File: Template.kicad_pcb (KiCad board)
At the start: 2 copper layers, 62 x 62 mm, 154 parts, among them J10 TAG, J20 TAG, J50 Goldpin, J60 RS232_Power, J61 RS232_Data, J70 USB, J84 Key, J86 Key, J87 Key, J90 12VIN, K85 CONFIG, T80 BC847, T81 BC847, T82 BC847, T83 BC847, T84 BC847, T90 BC847, U10 ATmega4809-MFR, U20 ATSAMW25-MR210PB, U30 ATECC608A-SSHDA, U31 ATECC608A-MAHDA, U40 GD25Q64C, U60 MAX3232, U70 FT230XQ, U90 AP3211, U91 1117-3.3, X10 32768Hz

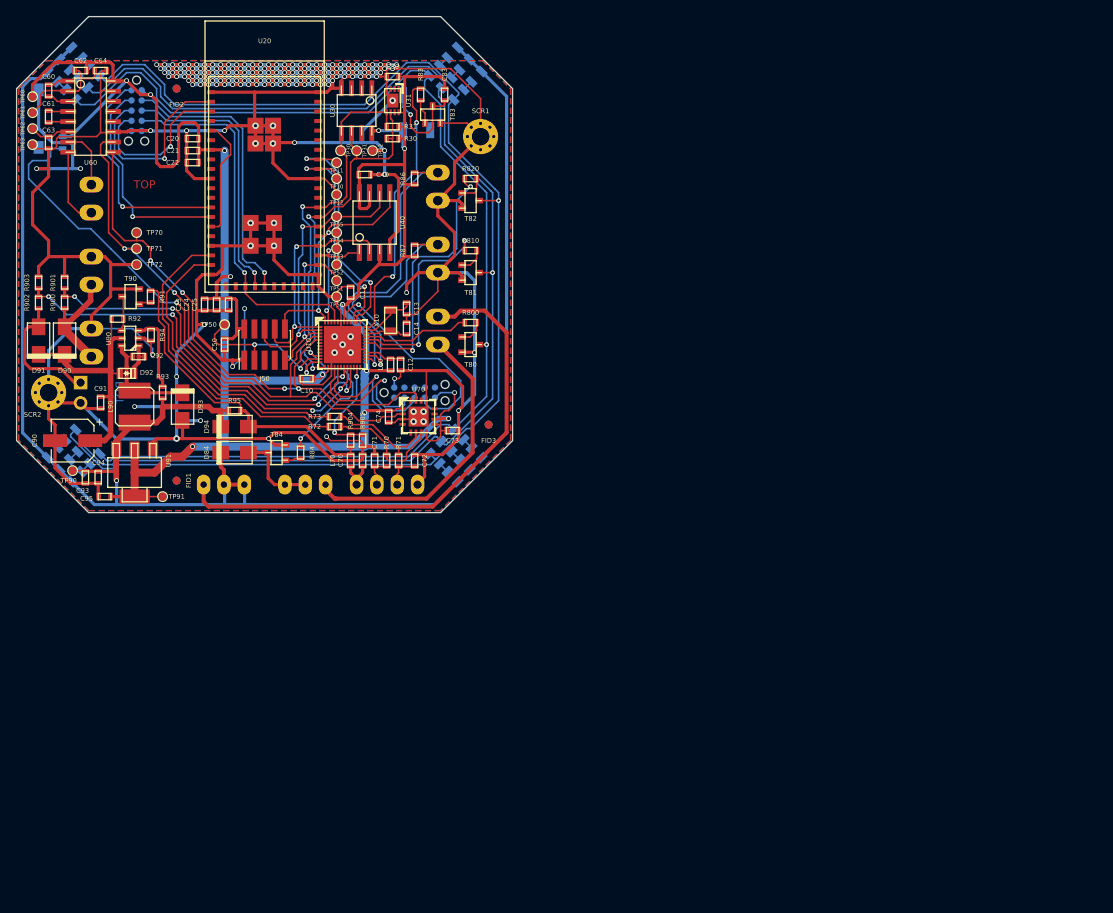
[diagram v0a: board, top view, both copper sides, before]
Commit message: Testowa modyfikacja
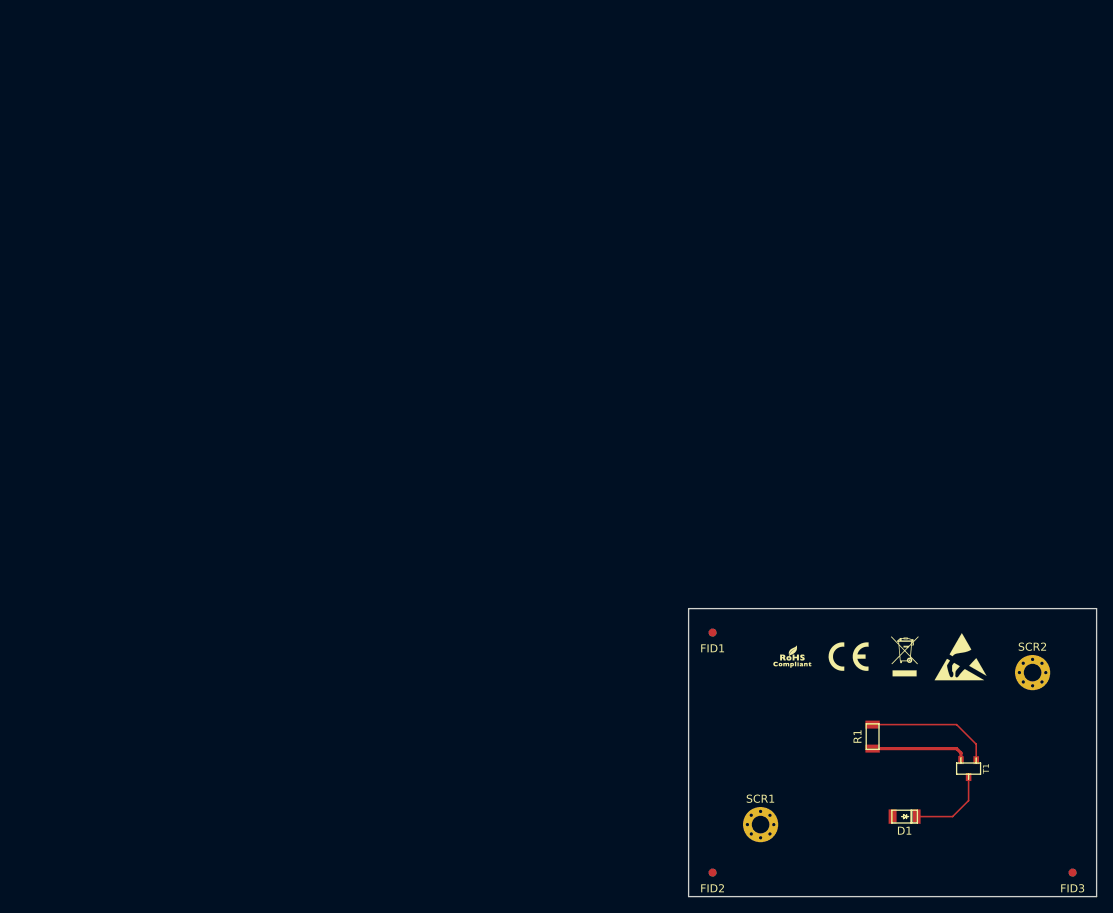
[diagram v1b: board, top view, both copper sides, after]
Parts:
- removed BT90: BATTERY, Pin_Headers:Pin_Header_Straight_1x02_Pitch2.54mm
- removed C10, C11, C12, C20, C23, C30, C50, C60, C61, C62, C63, C64, C70, C73, C74, C83, C94: 100n, _obudowy:C_0603
- removed C13, C14, C40: 15p, _obudowy:C_0603
- removed C21, C24: 1u, _obudowy:C_0603
- removed C22, C25, C93, C95: 10u, _obudowy:C_0603
- removed C71, C72: 22p, _obudowy:C_0603
- removed C90: 10u/50V, Capacitors_SMD:CP_Elec_5x5.8
- removed C91: 100n/50V, _obudowy:C_0603
- removed C92: 10n, _obudowy:C_0603
- removed D801, D802, D803, D804: Red, _obudowy:LED_0805
- removed D811, D812, D813, D814: Green, _obudowy:LED_0805
- removed D821, D822, D823, D824: Blue, _obudowy:LED_0805
- removed D84, D90, D91, D93, D94: SS14, _obudowy:D_SMA_DO214AC
- removed D92: 1N4148, _obudowy:D_0805
- removed G***: LOGO, _obudowy:SafliLogo
- removed J10, J20: TAG, _obudowy:TAG-TC2050
- removed J50: Goldpin, Pin_Headers:Pin_Header_Straight_2x05_Pitch1.27mm_SMD
- removed J60: RS232_Power, _obudowy:ADAM_TECH_EB59A-1-02-A-R
- removed J61: RS232_Data, _obudowy:ADAM_TECH_EB59A-1-02-A-R
- removed J70: USB, Pin_Headers:Pin_Header_Straight_1x04_Pitch2.54mm
- removed J84, J86, J87: Key, _obudowy:ADAM_TECH_EB59A-1-02-A-R
- removed J90: 12VIN, _obudowy:ADAM_TECH_EB59A-1-02-A-R
- removed K85: CONFIG, _obudowy:TACT_6x3.5_SMD
- removed L10, L70: BLM18PG471SN1, _obudowy:L_0603
- removed L90: 4.7uH, _obudowy:DJNR4018-5020
- removed R30, R31, R85, R86, R87, R901, R903, R904, R905, R91: 10k, _obudowy:R_0603
- removed R70, R71: 22R, _obudowy:R_0603
- removed R72, R73, R95: 0R, _obudowy:R_0603
- removed R800, R810, R820, R83, R84: 1k, _obudowy:R_0603
- removed R801, R802, R803, R804, R811, R812, R813, R814, R821, R822, R823, R824: 220R, _obudowy:R_0805
- removed R900, R902: 100k, _obudowy:R_0603
- removed R92: 1M, _obudowy:R_0603
- removed R93: 27k, _obudowy:R_0603
- removed R94: 5k1, _obudowy:R_0603
- removed RY80: RayexR1, _obudowy:Relay-Rayex1357
- removed S83: LD-BZEL-T54-0505, _obudowy:Loudity-SMT54
- removed T80, T81, T82, T83, T84, T90: BC847, _obudowy:SOT23
- removed TP10: LinkRx, _obudowy:Testpoint_1.00mm
- removed TP11: LinkTx, _obudowy:Testpoint_1.00mm
- removed TP12, TP32, TP56, TP63, TP72: GND, _obudowy:Testpoint_1.00mm
- removed TP30: SDA, _obudowy:Testpoint_1.00mm
- removed TP31: SCL, _obudowy:Testpoint_1.00mm
- removed TP50: Reset-RFID, _obudowy:Testpoint_1.00mm
- removed TP51: CS-RFID, _obudowy:Testpoint_1.00mm
- removed TP52: CS-Flash, _obudowy:Testpoint_1.00mm
- removed TP53: MISO, _obudowy:Testpoint_1.00mm
- removed TP54: MOSI, _obudowy:Testpoint_1.00mm
- removed TP55: SCK, _obudowy:Testpoint_1.00mm
- removed TP60: Vcc, _obudowy:Testpoint_1.00mm
- removed TP61: V+, _obudowy:Testpoint_1.00mm
- removed TP62: V-, _obudowy:Testpoint_1.00mm
- removed TP70: ComRx, _obudowy:Testpoint_1.00mm
- removed TP71: ComTx, _obudowy:Testpoint_1.00mm
- removed TP90: 5V, _obudowy:Testpoint_1.00mm
- removed TP91: 3V3, _obudowy:Testpoint_1.00mm
- removed U10: ATmega4809-MFR, _obudowy:QFN-48-1EP_6x6mm_Pitch0.4mm
- removed U20: ATSAMW25-MR210PB, _obudowy:SAMW25
- removed U30: ATECC608A-SSHDA, w_smd_dil:so-8
- removed U31: ATECC608A-MAHDA, _obudowy:DFN-8-1EP_3x2mm_Pitch0.5mm
- removed U40: GD25Q64C, w_smd_dil:soij-8
- removed U60: MAX3232, w_smd_dil:so-16
- removed U70: FT230XQ, _obudowy:QFN-16-1EP_4x4mm_Pitch0.65mm
- removed U90: AP3211, _obudowy:SOT23-6
- removed U91: 1117-3.3, _obudowy:SOT223
- removed X10: 32768Hz, _obudowy:Crystal_3.2x1.5
- added D1: LED, _obudowy:LED_1206, F.Cu at (131.0, 104.0)
- added R1: R, _obudowy:R_1206, F.Cu at (127.0, 94.0)
- added T1: BC847, _obudowy:SOT23, F.Cu at (139.0, 98.0)
- ICON1, ICON2, ICON3, ICON4: moved to F.Cu
- moved SCR2 127.9 mm to (147.0, 86.0)
- moved ICON2 123.5 mm to (131.0, 84.0), turned to 0 degrees
- moved FID2 118.7 mm to (107.0, 111.0)
- moved FID5 118.7 mm to (107.0, 111.0)
- moved ICON4 106.2 mm to (138.0, 84.0), turned to 0 degrees
- moved ICON1 95.6 mm to (124.0, 84.0), turned to 0 degrees
- moved SCR1 92.8 mm to (113.0, 105.0)
- moved FID3 92.0 mm to (152.0, 111.0)
- moved FID6 92.0 mm to (152.0, 111.0)
- moved FID1 69.6 mm to (107.0, 81.0)
- moved FID4 69.6 mm to (107.0, 81.0)
- moved ICON3 55.8 mm to (117.0, 84.0), turned to 0 degrees
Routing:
- net GND: track 719.1 -> 12.2 mm, vias 193 -> 0
- net 3V3: track 297.2 -> 0.00 mm, vias 13 -> 0
- net 5V: track 218.6 -> 0.00 mm, vias 1 -> 0
- net Net-(R821-Pad1): track 157.5 -> 0.00 mm, vias 1 -> 0
- net Net-(R811-Pad1): track 153.3 -> 0.00 mm, vias 1 -> 0
- net Net-(R801-Pad1): track 148.6 -> 0.00 mm, vias 1 -> 0
- net /AVR/Com-Tx: track 73.9 -> 0.00 mm, vias 2 -> 0
- net /AVR/Com-Rx: track 70.6 -> 0.00 mm, vias 4 -> 0
- net Net-(J84-Pad2): track 66.6 -> 0.00 mm
- net /AVR/Key-Config: track 64.5 -> 0.00 mm, vias 3 -> 0
- net /AVR/Volt-BAT: track 51.0 -> 0.00 mm, vias 4 -> 0
- net /AVR/I2C-SDA: track 49.7 -> 0.00 mm, vias 2 -> 0
- net /AVR/Volt-DC: track 49.3 -> 0.00 mm, vias 4 -> 0
- net /AVR/I2C-SCL: track 48.1 -> 0.00 mm, vias 2 -> 0
- net /AVR/SAM-Reset: track 46.3 -> 0.00 mm, vias 1 -> 0
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- removed copper zone on B.Cu, net GND
- removed copper zone on F.Cu, net GND
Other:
- board size 62 x 62 mm -> 51 x 36 mm
- board text removed: "-IN+"
- board text removed: "-OUT+"
- board text removed: "0"
- board text removed: "11"
- board text removed: "15"
- board text removed: "20"
- board text removed: "3"
- board text removed: "4"
- board text removed: "47"
- board text removed: "49"
- board text removed: "53"
- board text removed: "58"
- board text removed: "59"
- board text removed: "62"
- board text removed: "9"
- board text removed: "BOT"
- board text removed: "Halko v100"
- board text removed: "K-In"
- board text removed: "K-Out"
- board text removed: "Relay"
- board text removed: "SAFLI"
- board text removed: "TOP"
- board text removed: "Tx Rx"
